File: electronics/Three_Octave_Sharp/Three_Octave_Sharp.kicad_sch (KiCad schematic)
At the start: 108 parts, among them J1 HRO_TYPE-C-31-M-12, SW1 Key Tab, SW10 Key O, SW11 Key P, SW12 Key BS, SW16 Key Caps, SW17 Key A, SW18 Key S, SW19 Key D, SW2 Key Q, SW20 Key F, SW21 Alps_Alpine_SKRP, SW21 Key G, SW22 Alps_Alpine_SKRP, SW22 Key H, SW23 Key J, SW24 Key K, SW25 Key L, SW26 Key Return, SW3 Key W, SW30 Key Shift, SW31 Key Z, SW32 Key X, SW33 Key C, SW33 Key Shift, SW34 Key V, SW35 Key B, SW36 Key N, SW37 Key M, SW38 Key ,, SW4 Key E, SW43 Key Ctrl, SW44 Key Cmd, SW45 Key Space, SW46 Key Opt, SW47 Key Fn, SW5 Key R, SW6 Key T, SW7 Key Y, SW8 Key U, SW9 Key I, U1 AP2112K-3.3, U2 Raspberry_Pi_RP2040, U2 W25Q64JVXGIQ, Y1 12MHz

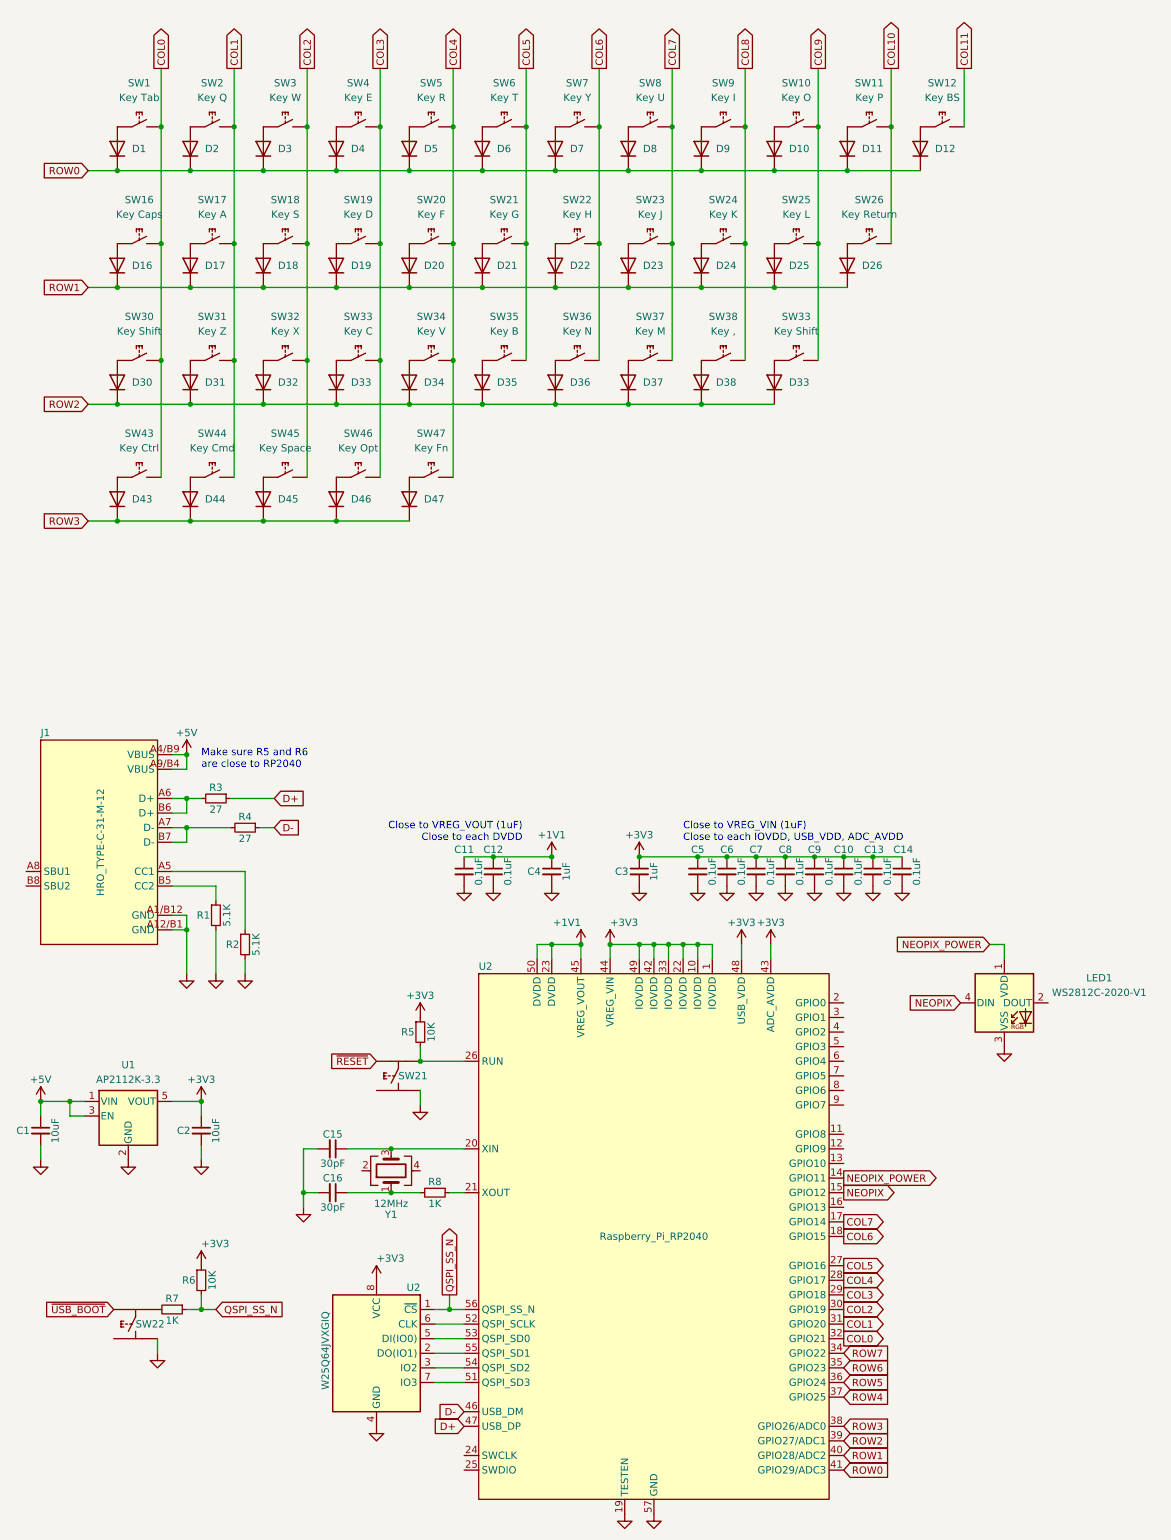
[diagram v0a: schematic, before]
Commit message: WIP: Update schematic and PCB design
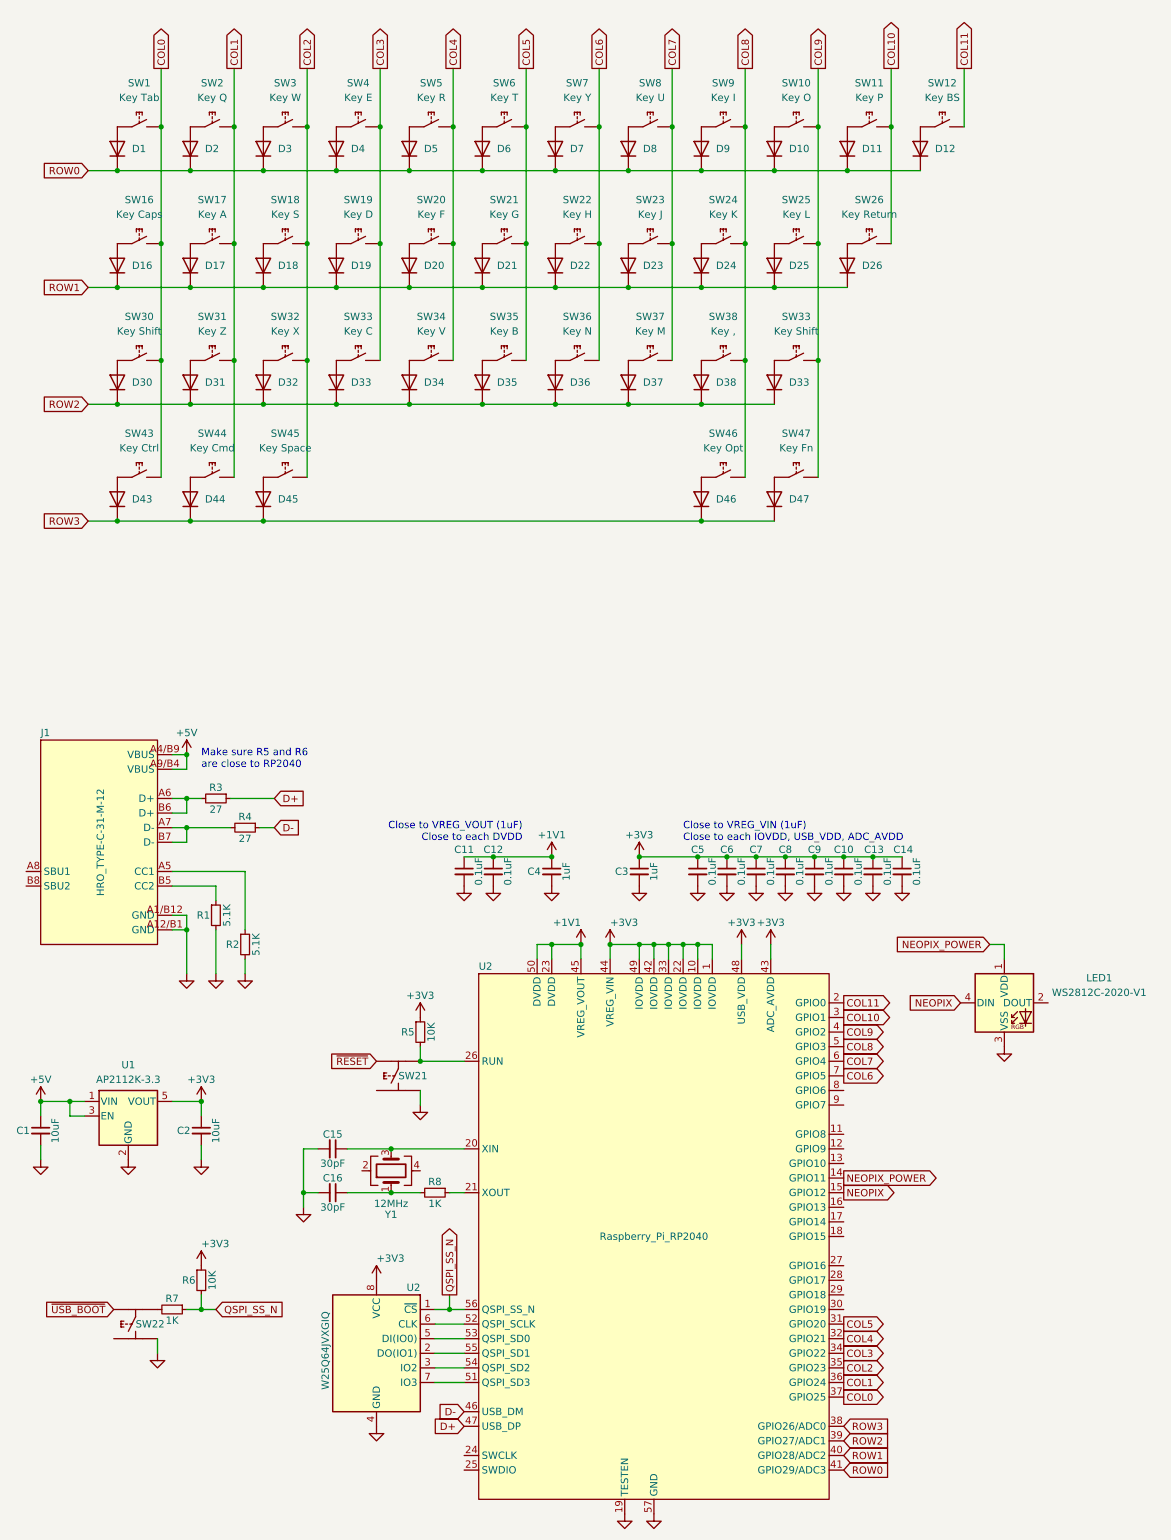
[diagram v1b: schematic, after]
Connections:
- net ROW4 is gone; now on net COL0: U2.37 (GPIO25)
- net ROW5 is gone; now on net COL1: U2.36 (GPIO24)
- net ROW6 is gone; now on net COL2: U2.35 (GPIO23)
- net ROW7 is gone; now on net COL3: U2.34 (GPIO22)
- net COL0: no longer U2.32 (GPIO21)
- net COL1: no longer U2.31 (GPIO20)
- net COL10: now also U2.3 (GPIO1)
- net COL11: now also U2.2 (GPIO0)
- net COL2: no longer U2.30 (GPIO19)
- net COL3: no longer SW46.2, U2.29 (GPIO18)
- net COL4: now also U2.32 (GPIO21); no longer SW47.2, U2.28 (GPIO17)
- net COL5: now also U2.31 (GPIO20); no longer U2.27 (GPIO16)
- net COL6: now also U2.7 (GPIO5); no longer U2.18 (GPIO15)
- net COL7: now also U2.6 (GPIO4); no longer U2.17 (GPIO14)
- net COL8: now also SW46.2, U2.5 (GPIO3)
- net COL9: now also SW47.2, U2.4 (GPIO2)
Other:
- moved on the sheet: D46, D47, SW46, SW47

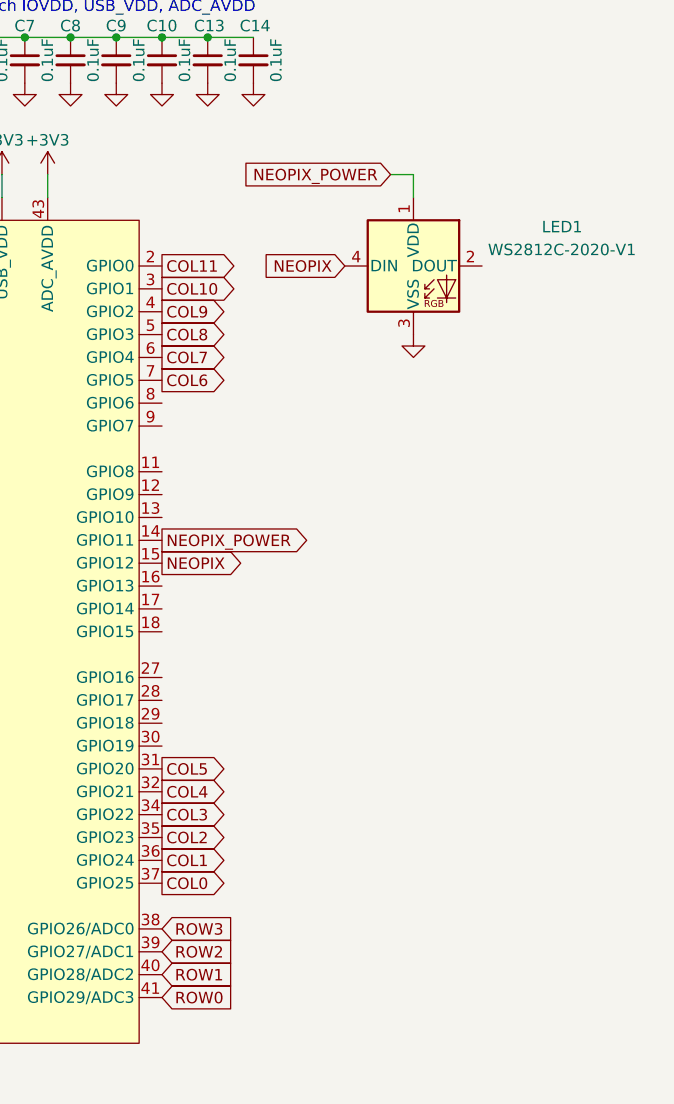
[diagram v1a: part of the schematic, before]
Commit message: WIP: Update schematic and PCB design
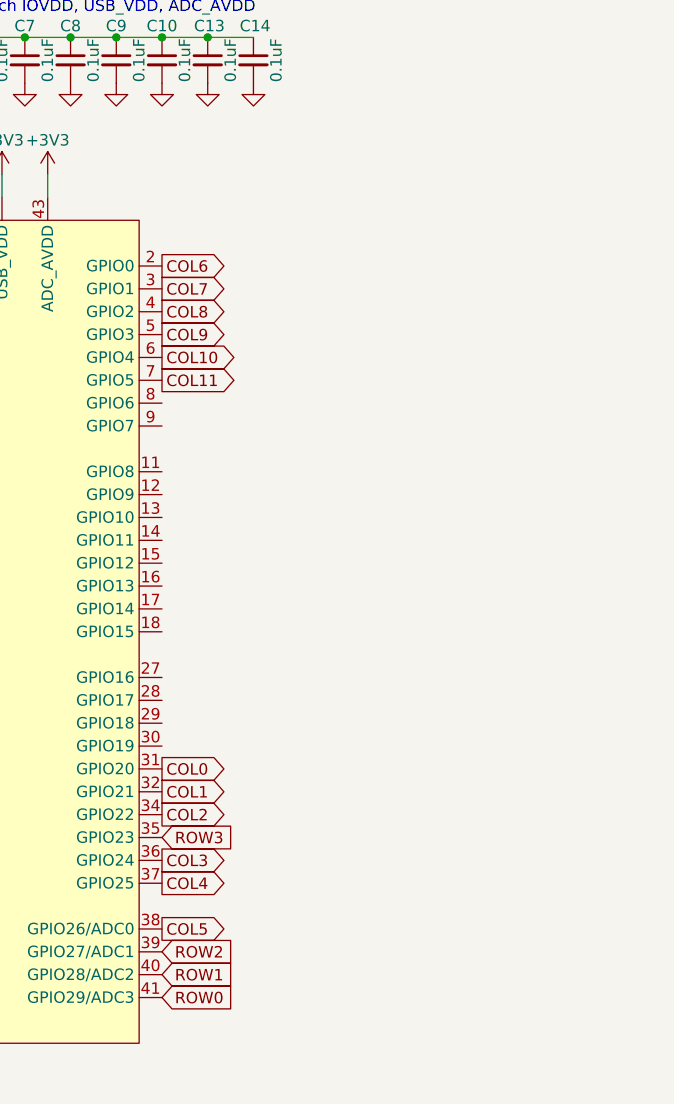
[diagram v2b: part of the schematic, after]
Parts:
- removed LED1: WS2812C-2020-V1, Project_Library:WS2812C-2020, symbol LED:WS2812B
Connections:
- net COL0: now also U2.31 (GPIO20); no longer U2.37 (GPIO25)
- net COL1: now also U2.32 (GPIO21); no longer U2.36 (GPIO24)
- net COL10: now also U2.6 (GPIO4); no longer U2.3 (GPIO1)
- net COL11: now also U2.7 (GPIO5); no longer U2.2 (GPIO0)
- net COL2: now also U2.34 (GPIO22); no longer U2.35 (GPIO23)
- net COL3: now also U2.36 (GPIO24); no longer U2.34 (GPIO22)
- net COL4: now also U2.37 (GPIO25); no longer U2.32 (GPIO21)
- net COL5: now also U2.38 (GPIO26/ADC0); no longer U2.31 (GPIO20)
- net COL6: now also U2.2 (GPIO0); no longer U2.7 (GPIO5)
- net COL7: now also U2.3 (GPIO1); no longer U2.6 (GPIO4)
- net COL8: now also U2.4 (GPIO2); no longer U2.5 (GPIO3)
- net COL9: now also U2.5 (GPIO3); no longer U2.4 (GPIO2)
- net ROW3: now also U2.35 (GPIO23); no longer U2.38 (GPIO26/ADC0)
- net NEOPIX: no longer names the net of U2.15 (GPIO12)
- net NEOPIX_POWER: no longer names the net of U2.14 (GPIO11)
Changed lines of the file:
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@@
     (stroke (width 0) (type default))
   )
-  (wire (pts (xy 187.325 177.8) (xy 189.865 177.8))
-    (stroke (width 0) (type default))
-  )
   (wire (pts (xy 47.625 175.26) (xy 47.625 182.88))
     (stroke (width 0) (type default))
@@
     (stroke (width 0) (type default))
   )
-  (wire (pts (xy 189.865 177.8) (xy 189.865 180.34))
-    (stroke (width 0) (type default))
-  )
   (wire (pts (xy 121.285 177.8) (xy 121.285 180.34))
     (stroke (width 0) (type default))
@@
     )
   )
-  (global_label "COL4" (shape output) (at 161.925 246.38 0) (fields_autoplaced)
+  (global_label "COL4" (shape output) (at 161.925 256.54 0) (fields_autoplaced)
     (effects (font (size 1.27 1.27)) (justify left))
-    (property "Intersheetrefs" "${INTERSHEET_REFS}" (at 169.7483 246.38 0)
+    (property "Intersheetrefs" "${INTERSHEET_REFS}" (at 169.7483 256.54 0)
       (effects (font (size 1.27 1.27)) (justify left) hide)
     )
   )
-  (global_label "COL6" (shape output) (at 161.925 200.66 0) (fields_autoplaced)
+  (global_label "COL6" (shape output) (at 161.925 187.96 0) (fields_autoplaced)
     (effects (font (size 1.27 1.27)) (justify left))
-    (property "Intersheetrefs" "${INTERSHEET_REFS}" (at 169.7483 200.66 0)
+    (property "Intersheetrefs" "${INTERSHEET_REFS}" (at 169.7483 187.96 0)
       (effects (font (size 1.27 1.27)) (justify left) hide)
     )
   )
-  (global_label "ROW3" (shape input) (at 161.925 261.62 0) (fields_autoplaced)
+  (global_label "ROW3" (shape input) (at 161.925 251.46 0) (fields_autoplaced)
     (effects (font (size 1.27 1.27)) (justify left))
-    (property "Intersheetrefs" "${INTERSHEET_REFS}" (at 170.1716 261.62 0)
+    (property "Intersheetrefs" "${INTERSHEET_REFS}" (at 170.1716 251.46 0)
       (effects (font (size 1.27 1.27)) (justify left) hide)
     )
@@
     )
   )
-  (global_label "NEOPIX" (shape output) (at 161.925 220.98 0) (fields_autoplaced)
-    (effects (font (size 1.27 1.27)) (justify left))
-    (property "Intersheetrefs" "${INTERSHEET_REFS}" (at 171.2324 220.9006 0)
-      (effects (font (size 1.27 1.27)) (justify left) hide)
-    )
-  )
   (global_label "~{USB_BOOT}" (shape input) (at 34.925 241.3 180) (fields_autoplaced)
     (effects (font (size 1.27 1.27)) (justify right))
@@
     )
   )
-  (global_label "NEOPIX" (shape input) (at 182.245 187.96 180) (fields_autoplaced)
-    (effects (font (size 1.27 1.27)) (justify right))
-    (property "Intersheetrefs" "${INTERSHEET_REFS}" (at 172.9376 188.0394 0)
-      (effects (font (size 1.27 1.27)) (justify right) hide)
-    )
-  )
-  (global_label "COL8" (shape output) (at 161.925 195.58 0) (fields_autoplaced)
+  (global_label "COL8" (shape output) (at 161.925 193.04 0) (fields_autoplaced)
     (effects (font (size 1.27 1.27)) (justify left))
-    (property "Intersheetrefs" "${INTERSHEET_REFS}" (at 169.7483 195.58 0)
+    (property "Intersheetrefs" "${INTERSHEET_REFS}" (at 169.7483 193.04 0)
       (effects (font (size 1.27 1.27)) (justify left) hide)
     )
@@
     )
   )
-  (global_label "COL2" (shape output) (at 161.925 251.46 0) (fields_autoplaced)
+  (global_label "COL2" (shape output) (at 161.925 248.92 0) (fields_autoplaced)
     (effects (font (size 1.27 1.27)) (justify left))
-    (property "Intersheetrefs" "${INTERSHEET_REFS}" (at 169.7483 251.46 0)
+    (property "Intersheetrefs" "${INTERSHEET_REFS}" (at 169.7483 248.92 0)
       (effects (font (size 1.27 1.27)) (justify left) hide)
     )
@@
     )
   )
-  (global_label "COL9" (shape output) (at 161.925 193.04 0) (fields_autoplaced)
+  (global_label "COL9" (shape output) (at 161.925 195.58 0) (fields_autoplaced)
     (effects (font (size 1.27 1.27)) (justify left))
-    (property "Intersheetrefs" "${INTERSHEET_REFS}" (at 169.7483 193.04 0)
+    (property "Intersheetrefs" "${INTERSHEET_REFS}" (at 169.7483 195.58 0)
       (effects (font (size 1.27 1.27)) (justify left) hide)
     )
   )
-  (global_label "COL10" (shape output) (at 161.925 190.5 0) (fields_autoplaced)
+  (global_label "COL10" (shape output) (at 161.925 198.12 0) (fields_autoplaced)
     (effects (font (size 1.27 1.27)) (justify left))
-    (property "Intersheetrefs" "${INTERSHEET_REFS}" (at 170.9578 190.5 0)
+    (property "Intersheetrefs" "${INTERSHEET_REFS}" (at 170.9578 198.12 0)
       (effects (font (size 1.27 1.27)) (justify left) hide)
     )
@@
     )
   )
-  (global_label "COL1" (shape output) (at 161.925 254 0) (fields_autoplaced)
+  (global_label "COL1" (shape output) (at 161.925 246.38 0) (fields_autoplaced)
     (effects (font (size 1.27 1.27)) (justify left))
-    (property "Intersheetrefs" "${INTERSHEET_REFS}" (at 169.7483 254 0)
+    (property "Intersheetrefs" "${INTERSHEET_REFS}" (at 169.7483 246.38 0)
       (effects (font (size 1.27 1.27)) (justify left) hide)
     )
   )
-  (global_label "COL5" (shape output) (at 161.925 243.84 0) (fields_autoplaced)
+  (global_label "COL5" (shape output) (at 161.925 261.62 0) (fields_autoplaced)
     (effects (font (size 1.27 1.27)) (justify left))
-    (property "Intersheetrefs" "${INTERSHEET_REFS}" (at 169.7483 243.84 0)
+    (property "Intersheetrefs" "${INTERSHEET_REFS}" (at 169.7483 261.62 0)
       (effects (font (size 1.27 1.27)) (justify left) hide)
     )
   )
-  (global_label "COL11" (shape output) (at 161.925 187.96 0) (fields_autoplaced)
+  (global_label "COL11" (shape output) (at 161.925 200.66 0) (fields_autoplaced)
     (effects (font (size 1.27 1.27)) (justify left))
-    (property "Intersheetrefs" "${INTERSHEET_REFS}" (at 170.9578 187.96 0)
+    (property "Intersheetrefs" "${INTERSHEET_REFS}" (at 170.9578 200.66 0)
       (effects (font (size 1.27 1.27)) (justify left) hide)
     )
@@
     )
   )
-  (global_label "NEOPIX_POWER" (shape input) (at 187.325 177.8 180) (fields_autoplaced)
-    (effects (font (size 1.27 1.27)) (justify right))
-    (property "Intersheetrefs" "${INTERSHEET_REFS}" (at 170.007 177.8 0)
-      (effects (font (size 1.27 1.27)) (justify right) hide)
-    )
-  )
   (global_label "COL1" (shape output) (at 55.88 25.4 90) (fields_autoplaced)
     (effects (font (size 1.27 1.27)) (justify left))
@@
     )
   )
-  (global_label "COL3" (shape output) (at 161.925 248.92 0) (fields_autoplaced)
+  (global_label "COL3" (shape output) (at 161.925 254 0) (fields_autoplaced)
     (effects (font (size 1.27 1.27)) (justify left))
-    (property "Intersheetrefs" "${INTERSHEET_REFS}" (at 169.7483 248.92 0)
+    (property "Intersheetrefs" "${INTERSHEET_REFS}" (at 169.7483 254 0)
       (effects (font (size 1.27 1.27)) (justify left) hide)
     )
@@
     )
   )
-  (global_label "COL0" (shape output) (at 161.925 256.54 0) (fields_autoplaced)
-    (effects (font (size 1.27 1.27)) (justify left))
-    (property "Intersheetrefs" "${INTERSHEET_REFS}" (at 169.7483 256.54 0)
-      (effects (font (size 1.27 1.27)) (justify left) hide)
-    )
-  )
-  (global_label "NEOPIX_POWER" (shape output) (at 161.925 218.44 0) (fields_autoplaced)
+  (global_label "COL0" (shape output) (at 161.925 243.84 0) (fields_autoplaced)
     (effects (font (size 1.27 1.27)) (justify left))
-    (property "Intersheetrefs" "${INTERSHEET_REFS}" (at 178.671 218.3606 0)
+    (property "Intersheetrefs" "${INTERSHEET_REFS}" (at 169.7483 243.84 0)
       (effects (font (size 1.27 1.27)) (justify left) hide)
     )
   )
-  (global_label "COL7" (shape output) (at 161.925 198.12 0) (fields_autoplaced)
+  (global_label "COL7" (shape output) (at 161.925 190.5 0) (fields_autoplaced)
     (effects (font (size 1.27 1.27)) (justify left))
-    (property "Intersheetrefs" "${INTERSHEET_REFS}" (at 169.7483 198.12 0)
+    (property "Intersheetrefs" "${INTERSHEET_REFS}" (at 169.7483 190.5 0)
       (effects (font (size 1.27 1.27)) (justify left) hide)
     )
@@
     )
   )
-  (symbol (lib_id "power:GND") (at 189.865 195.58 0) (unit 1)
-    (in_bom yes) (on_board yes) (dnp no) (fields_autoplaced)
-    (property "Reference" "#PWR0144" (at 189.865 201.93 0)
-      (effects (font (size 1.27 1.27)) hide)
-    )
-    (property "Value" "GND" (at 189.865 200.66 0)
-      (effects (font (size 1.27 1.27)) hide)
-    )
-    (property "Footprint" "" (at 189.865 195.58 0)
-      (effects (font (size 1.27 1.27)) hide)
-    )
-    (property "Datasheet" "" (at 189.865 195.58 0)
-      (effects (font (size 1.27 1.27)) hide)
-    )
-    (pin "1")
-    (instances
-      (project "Octave_Input_PCB"
-        (path "/8fd6d03b-a222-44f4-a556-6ddea29b94bc"
-          (reference "#PWR0144") (unit 1)
-        )
-      )
-      (project "Three_Octave_Sharp"
-        (path "/be77d40c-b3e5-4e63-afb1-cedcaf2c38de"
-          (reference "#PWR041") (unit 1)
-        )
-      )
-    )
-  )
   (symbol (lib_id "Device:C_Small") (at 111.125 165.1 0) (unit 1)
     (in_bom yes) (on_board yes) (dnp no)
@@
         )
       )
-    )
-  )
-  (symbol (lib_id "LED:WS2812B") (at 189.865 187.96 0) (unit 1)
-    (in_bom yes) (on_board yes) (dnp no)
-    (property "Reference" "LED1" (at 206.375 183.6293 0)
-      (effects (font (size 1.27 1.27)))
-    )
-    (property "Value" "WS2812C-2020-V1" (at 206.375 186.1693 0)
-      (effects (font (size 1.27 1.27)))
-    )
-    (property "Footprint" "Project_Library:WS2812C-2020" (at 191.135 195.58 0)
-      (effects (font (size 1.27 1.27)) (justify left top) hide)
-    )
-    (property "Datasheet" "" (at 192.405 197.485 0)
-      (effects (font (size 1.27 1.27)) (justify left top) hide)
-    )
-    (property "LCSC" "C2976072" (at 189.865 187.96 0)
-      (effects (font (size 1.27 1.27)) hide)
-    )
-    (pin "1")
-    (pin "2")
-    (pin "3")
-    (pin "4")
-    (instances
-      (project "Octave_Input_PCB"
-        (path "/8fd6d03b-a222-44f4-a556-6ddea29b94bc"
-          (reference "LED1") (unit 1)
-        )
-      )
-      (project "Three_Octave_Sharp"
-        (path "/be77d40c-b3e5-4e63-afb1-cedcaf2c38de"
-          (reference "LED1") (unit 1)
-        )
-      )
